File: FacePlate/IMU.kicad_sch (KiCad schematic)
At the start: 8 parts, among them U3 ICM-20689

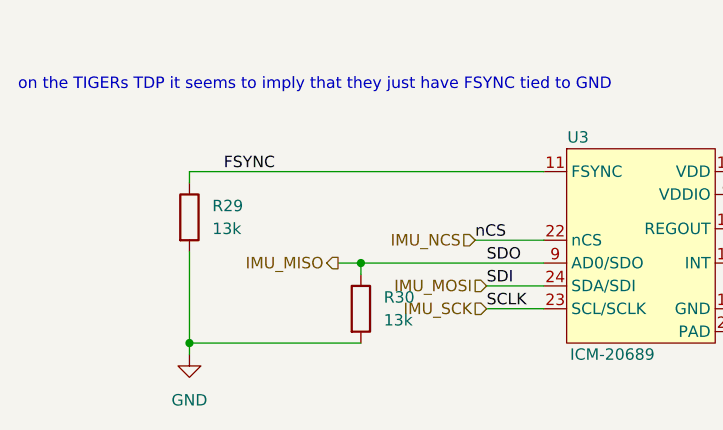
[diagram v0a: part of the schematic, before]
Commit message: faceplate global files working
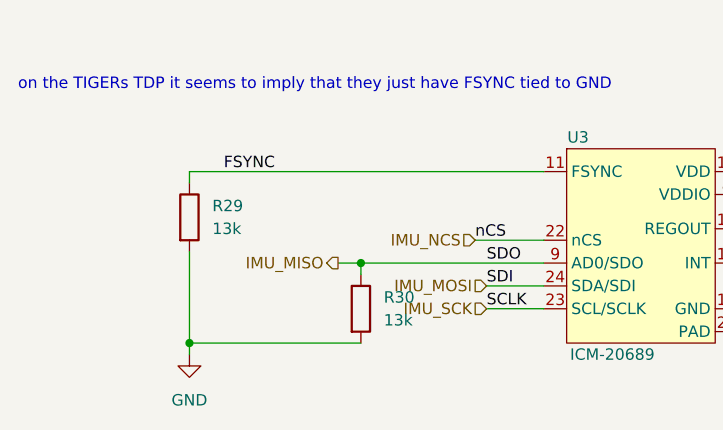
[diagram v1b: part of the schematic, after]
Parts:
- C14, C7: footprint bots:C_0603_1608Metric -> bots:C_0805_2012Metric; symbol Device:C -> bots:C_10u; JLC (none) -> 0805; JLC Extended (none) -> no; LCSC C96446 -> C440198; MPN (none) -> GRM21BR61H106KE43L; Manufacturer (none) -> Murata; Price (none) -> 0.0645
- R29, R30: symbol bots:10k -> bots:R_13k; JLC (none) -> 0603; JLC Extended (none) -> no; MPN (none) -> 0603WAF1302T5E; Manufacturer (none) -> UNI-ROYAL(Uniroyal Elec); Price (none) -> 0.0008
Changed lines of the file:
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@@
 	)
 	(symbol
-		(lib_id "Device:C")
+		(lib_id "bots:C_10u")
 		(at 143.51 69.85 0)
 		(unit 1)
@@
 			)
 		)
-		(property "Footprint" "bots:C_0603_1608Metric"
+		(property "Footprint" "bots:C_0805_2012Metric"
 			(at 144.4752 73.66 0)
 			(effects
@@
 			)
 		)
-		(property "Description" ""
+		(property "Description" "Unpolarized capacitor"
 			(at 143.51 69.85 0)
 			(effects
@@
 					(size 1.27 1.27)
 				)
-			)
-		)
-		(property "LCSC" "C96446"
+				(hide yes)
+			)
+		)
+		(property "LCSC" "C440198"
+			(at 143.51 69.85 0)
+			(effects
+				(font
+					(size 1.27 1.27)
+				)
+				(hide yes)
+			)
+		)
+		(property "MPN" "GRM21BR61H106KE43L"
+			(at 143.51 69.85 0)
+			(effects
+				(font
+					(size 1.27 1.27)
+				)
+				(hide yes)
+			)
+		)
+		(property "Manufacturer" "Murata"
+			(at 143.51 69.85 0)
+			(effects
+				(font
+					(size 1.27 1.27)
+				)
+				(hide yes)
+			)
+		)
+		(property "Price" "0.0645"
+			(at 143.51 69.85 0)
+			(effects
+				(font
+					(size 1.27 1.27)
+				)
+				(hide yes)
+			)
+		)
+		(property "JLC" "0805"
+			(at 143.51 69.85 0)
+			(effects
+				(font
+					(size 1.27 1.27)
+				)
+				(hide yes)
+			)
+		)
+		(property "JLC Extended" "no"
 			(at 143.51 69.85 0)
 			(effects
@@
 	)
 	(symbol
-		(lib_id "bots:10k")
+		(lib_id "bots:R_13k")
 		(at 58.42 74.93 0)
 		(unit 1)
@@
 		(fields_autoplaced yes)
 		(property "Reference" "R30"
-			(at 60.96 73.66 0)
+			(at 60.96 73.6599 0)
 			(effects
 				(font
@@
 		)
 		(property "Value" "13k"
-			(at 60.96 76.2 0)
+			(at 60.96 76.1999 0)
 			(effects
 				(font
@@
 			)
 		)
-		(property "Description" ""
+		(property "Description" "Resistor"
 			(at 58.42 74.93 0)
 			(effects
@@
 					(size 1.27 1.27)
 				)
+				(hide yes)
 			)
 		)
 		(property "LCSC" "C22797"
+			(at 58.42 74.93 0)
+			(effects
+				(font
+					(size 1.27 1.27)
+				)
+				(hide yes)
+			)
+		)
+		(property "MPN" "0603WAF1302T5E"
+			(at 58.42 74.93 0)
+			(effects
+				(font
+					(size 1.27 1.27)
+				)
+				(hide yes)
+			)
+		)
+		(property "Manufacturer" "UNI-ROYAL(Uniroyal Elec)"
+			(at 58.42 74.93 0)
+			(effects
+				(font
+					(size 1.27 1.27)
+				)
+				(hide yes)
+			)
+		)
+		(property "Price" "0.0008"
+			(at 58.42 74.93 0)
+			(effects
+				(font
+					(size 1.27 1.27)
+				)
+				(hide yes)
+			)
+		)
+		(property "JLC" "0603"
+			(at 58.42 74.93 0)
+			(effects
+				(font
+					(size 1.27 1.27)
+				)
+				(hide yes)
+			)
+		)
+		(property "JLC Extended" "no"
 			(at 58.42 74.93 0)
 			(effects
@@
 	)
 	(symbol
-		(lib_id "bots:10k")
+		(lib_id "bots:R_13k")
 		(at 39.37 64.77 0)
 		(unit 1)
@@
 		(fields_autoplaced yes)
 		(property "Reference" "R29"
-			(at 41.91 63.5 0)
+			(at 41.91 63.4999 0)
 			(effects
 				(font
@@
 		)
 		(property "Value" "13k"
-			(at 41.91 66.04 0)
+			(at 41.91 66.0399 0)
 			(effects
 				(font
@@
 			)
 		)
-		(property "Description" ""
+		(property "Description" "Resistor"
 			(at 39.37 64.77 0)
 			(effects
@@
 					(size 1.27 1.27)
 				)
+				(hide yes)
 			)
 		)
 		(property "LCSC" "C22797"
+			(at 39.37 64.77 0)
+			(effects
+				(font
+					(size 1.27 1.27)
+				)
+				(hide yes)
+			)
+		)
+		(property "MPN" "0603WAF1302T5E"
+			(at 39.37 64.77 0)
+			(effects
+				(font
+					(size 1.27 1.27)
+				)
+				(hide yes)
+			)
+		)
+		(property "Manufacturer" "UNI-ROYAL(Uniroyal Elec)"
+			(at 39.37 64.77 0)
+			(effects
+				(font
+					(size 1.27 1.27)
+				)
+				(hide yes)
+			)
+		)
+		(property "Price" "0.0008"
+			(at 39.37 64.77 0)
+			(effects
+				(font
+					(size 1.27 1.27)
+				)
+				(hide yes)
+			)
+		)
+		(property "JLC" "0603"
+			(at 39.37 64.77 0)
+			(effects
+				(font
+					(size 1.27 1.27)
+				)
+				(hide yes)
+			)
+		)
+		(property "JLC Extended" "no"
 			(at 39.37 64.77 0)
 			(effects
@@
 	)
 	(symbol
-		(lib_id "Device:C")
+		(lib_id "bots:C_10u")
 		(at 119.38 69.85 0)
 		(unit 1)
@@
 			)
 		)
-		(property "Footprint" "bots:C_0603_1608Metric"
+		(property "Footprint" "bots:C_0805_2012Metric"
 			(at 120.3452 73.66 0)
 			(effects
@@
 			)
 		)
-		(property "Description" ""
+		(property "Description" "Unpolarized capacitor"
 			(at 119.38 69.85 0)
 			(effects
@@
 					(size 1.27 1.27)
 				)
-			)
-		)
-		(property "LCSC" "C96446"
+				(hide yes)
+			)
+		)
+		(property "LCSC" "C440198"
 			(at 119.38 69.85 0)
 			(effects
+				(font
+					(size 1.27 1.27)
+				)
+				(hide yes)
+			)
+		)
+		(property "MPN" "GRM21BR61H106KE43L"
+			(at 119.38 69.85 0)
+			(effects
+				(font
+					(size 1.27 1.27)
+				)
+				(hide yes)
+			)
+		)
+		(property "Manufacturer" "Murata"
+			(at 119.38 69.85 0)
+			(effects
+				(font
+					(size 1.27 1.27)
+				)
+				(hide yes)
+			)
+		)
+		(property "Price" "0.0645"
+			(at 119.38 69.85 0)
+			(effects
+				(font
+					(size 1.27 1.27)
+				)
+				(hide yes)
+			)
+		)
+		(property "JLC" "0805"
+			(at 119.38 69.85 0)
+			(effects
+				(font
+					(size 1.27 1.27)
+				)
+				(hide yes)
+			)
+		)
+		(property "JLC Extended" "no"
+			(at 119.38 69.85 0)
+			(effects
